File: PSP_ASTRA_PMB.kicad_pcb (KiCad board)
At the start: 4 copper layers, 15 parts, among them J1 Conn_01x02_Socket, J2 Conn_01x01_Socket, J3 Screw_Terminal_01x03, J5 Screw_Terminal_01x01, J6 Screw_Terminal_01x01, Q1 BSC014N04LSIATMA1, U1 INA226, U5 LD1117V33

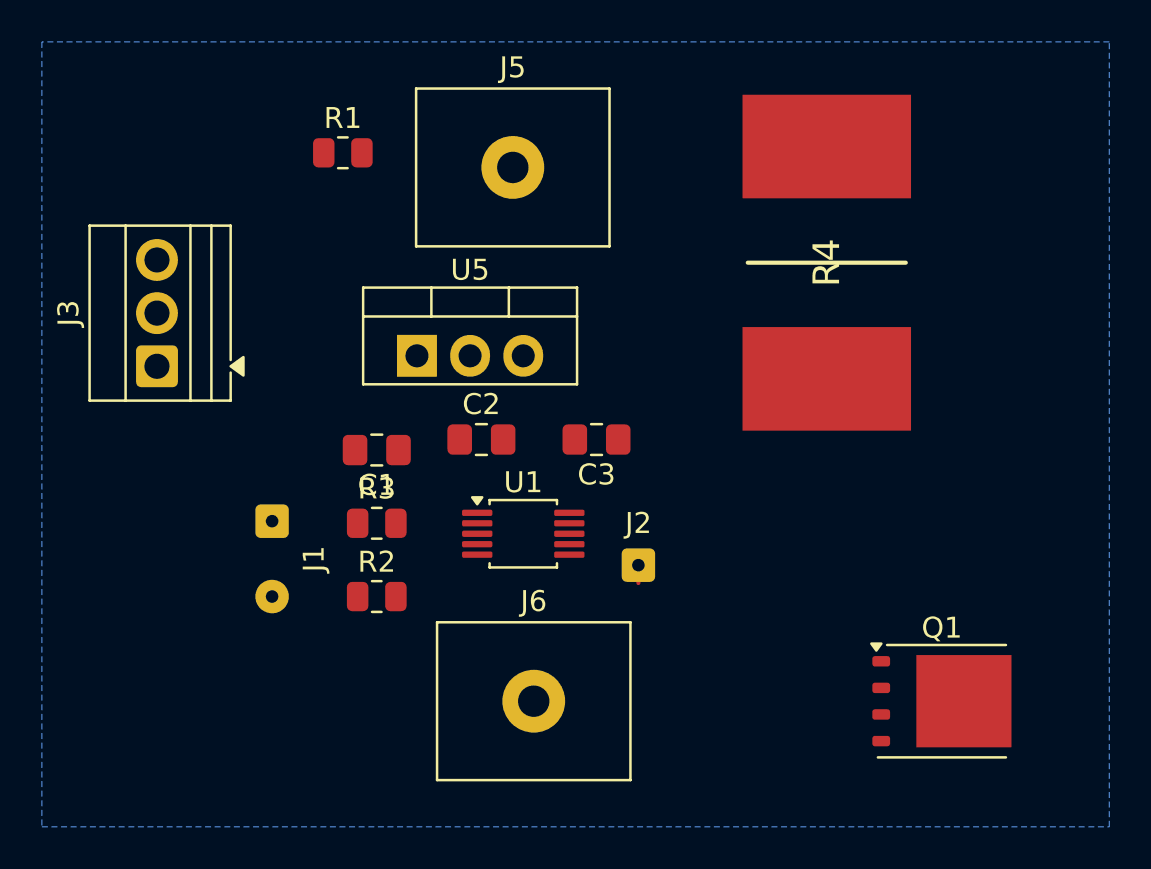
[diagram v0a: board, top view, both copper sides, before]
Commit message: Add files via upload
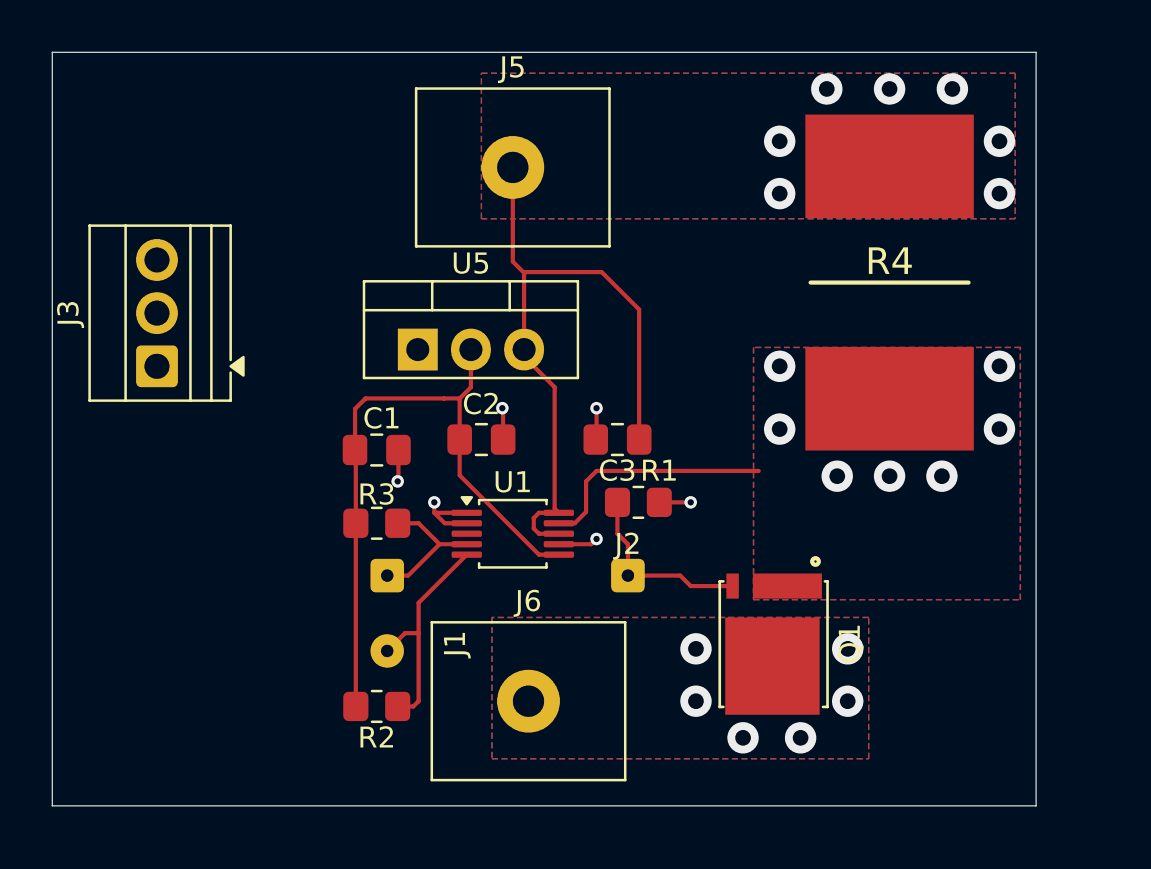
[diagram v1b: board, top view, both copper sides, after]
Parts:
- Q1: footprint Package_TO_SOT_SMD:TDSON-8-1 -> PSPAC:MOSFETPMB
- R1, R2, R3: footprint Resistor_SMD:R_0805_2012Metric -> Resistor_SMD:R_0805_2012Metric_Pad1.20x1.40mm_HandSolder
- moved R1 21.9 mm to (156.0, 100.5)
- moved Q1 8.49 mm to (162.5, 107.3), turned to -90 degrees
- moved J1 6.08 mm to (144.0, 104.0)
- moved R2 5.25 mm to (143.5, 110.2)
- moved R4 3.15 mm to (168.0, 90.0)
- moved C3 1.00 mm to (155.0, 97.5)
- moved J2 0.71 mm to (155.5, 104.0)
- moved U1 0.50 mm to (150.0, 102.0)
- moved U5 0.30 mm to (145.5, 93.2)
- moved J6 0.25 mm to (150.8, 110.0)
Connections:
- net Net-(Q1-D) renamed /Drain
- J6 pad 1: Net-(J6-Pin_1) -> /Source
- Q1 pad 4: (no net) -> /Microcontroller
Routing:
- net +12V: track 0.00 -> 33.7 mm, vias 0 -> 7
- net Net-(U1-VS): track 0.00 -> 32.0 mm
- net GND: track 0.00 -> 11.8 mm, vias 0 -> 6
- net /Drain: track 0.00 -> 11.4 mm, vias 0 -> 7
- net Net-(J1-Pin_2): track 0.00 -> 10.9 mm
- net /Microcontroller: track 0.85 -> 8.91 mm
- net Net-(J1-Pin_1): track 0.00 -> 6.84 mm
- net /Source: vias 0 -> 6
- added copper zone on B.Cu, net +12V
- added copper zone on F.Cu, net +12V
- added copper zone on In1.Cu, net +12V
- added copper zone on In2.Cu, net +12V
- added copper zone on B.Cu, net /Drain
- added copper zone on F.Cu, net /Drain
- added copper zone on In1.Cu, net /Drain
- added copper zone on In2.Cu, net /Drain
- added copper zone on B.Cu, net /Source
- added copper zone on F.Cu, net /Source
- added copper zone on In1.Cu, net /Source
- added copper zone on In2.Cu, net /Source
- added copper zone on In1.Cu, net GND
- removed copper zone on B.Cu, net GND
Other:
- board outline added: 47 x 36 mm
